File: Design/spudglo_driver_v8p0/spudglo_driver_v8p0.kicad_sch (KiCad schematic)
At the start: 25 parts, among them J3 terminal_custom_12pin, U1 rf_433MHz_module, U12 USB-C-31-M-12, U13 XR21B1411, U14 NCP361, U2 rf_433MHz_module, U3 rf_433MHz_module, U4 rf_433MHz_module

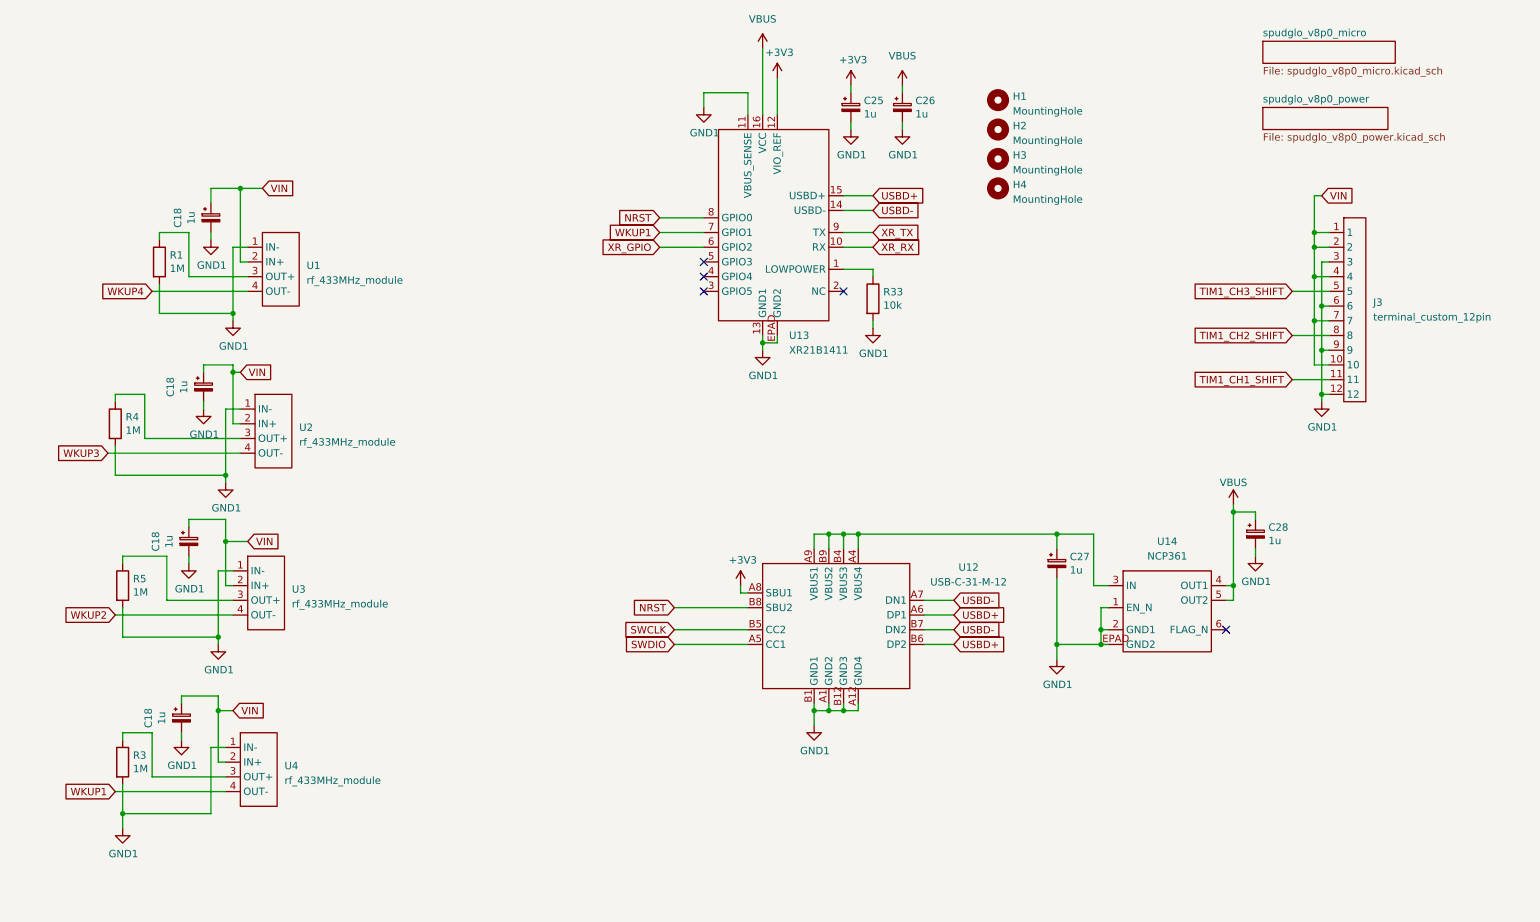
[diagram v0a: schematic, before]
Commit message: khg
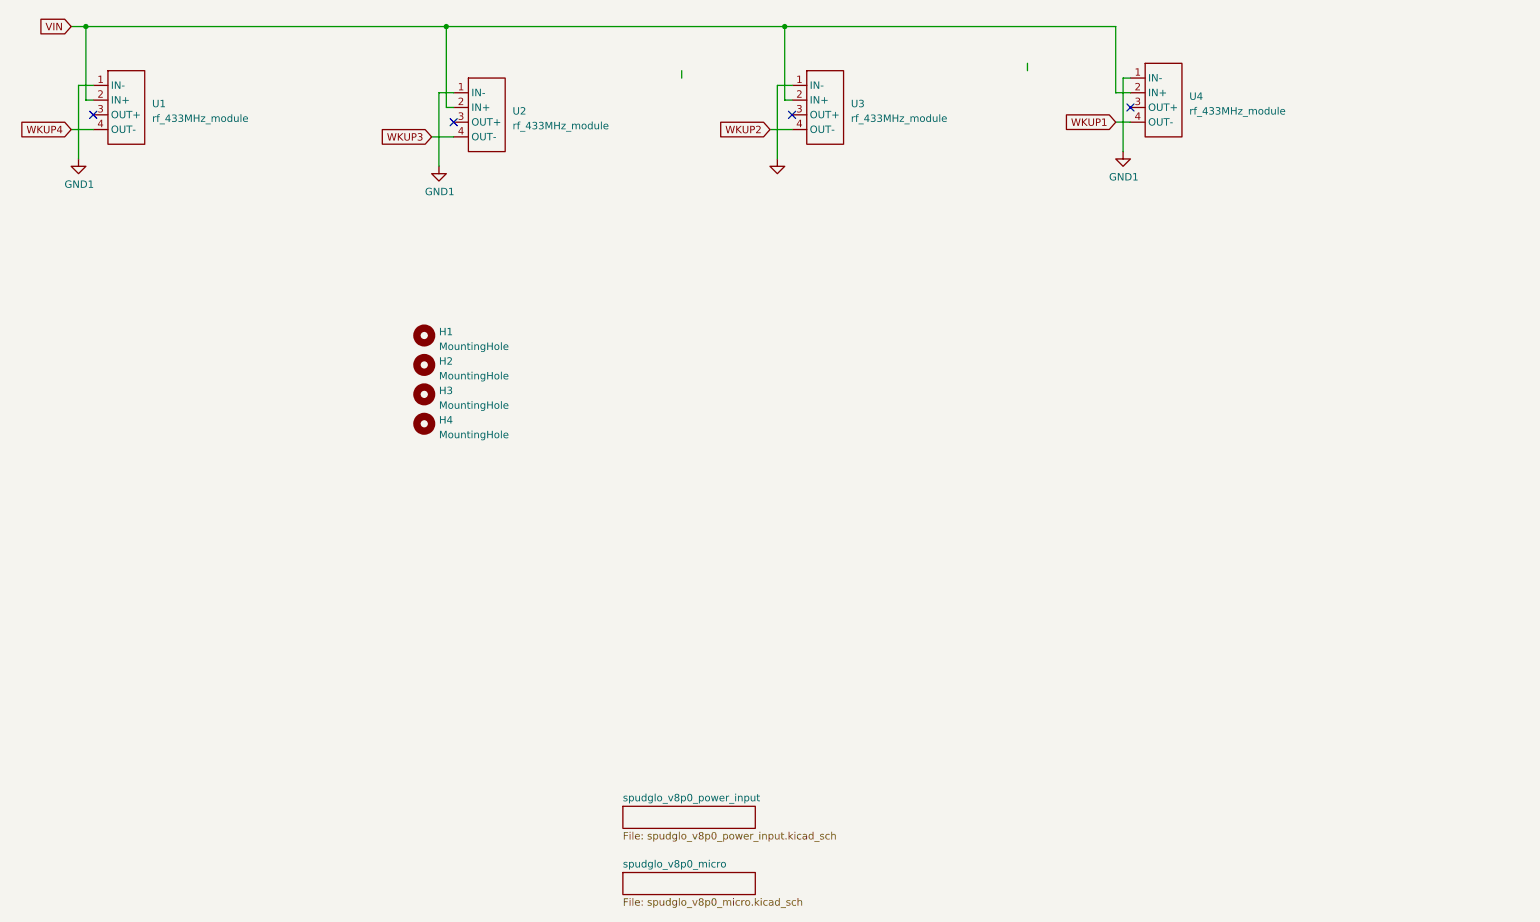
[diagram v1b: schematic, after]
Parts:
- removed C18 (x4), C25, C26, C27, C28: 1u, Capacitor_SMD:C_0402_1005Metric_Pad0.74x0.62mm_HandSolder, symbol spudglo_driver_v3p1-rescue:CP_Small-Device
- removed J3: terminal_custom_12pin, srw_custom:1984714, symbol srw_custom:terminal_custom_12pin
- removed R1, R3, R4, R5: 1M, Resistor_SMD:R_0402_1005Metric_Pad0.72x0.64mm_HandSolder, symbol Device:R
- removed R33: 10k, Resistor_SMD:R_0603_1608Metric_Pad0.98x0.95mm_HandSolder, symbol Device:R
- removed U12: USB-C-31-M-12, Connector_USB:USB_C_Receptacle_HRO_TYPE-C-31-M-12, symbol srw_custom:USB-C-31-M-12
- removed U13: XR21B1411, srw_cuustom:XR21B1411, symbol srw_custom:XR21B1411
- removed U14: NCP361, srw_cuustom:NCP361, symbol srw_custom:NCP361
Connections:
- no-connect marks 5 -> 4
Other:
- removed sheet spudglo_v8p0_power
- added sheet spudglo_v8p0_power_input (spudglo_v8p0_power_input.kicad_sch)
- moved on the sheet: U1, U2, U3, U4
